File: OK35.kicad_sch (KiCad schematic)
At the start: 74 parts, among them SW1 SW_SPST, SW10 SW_SPST, SW11 SW_SPST, SW12 SW_SPST, SW13 SW_SPST, SW14 SW_SPST, SW15 SW_SPST, SW16 SW_SPST, SW17 SW_SPST, SW18 SW_SPST, SW19 SW_SPST, SW2 SW_SPST, SW20 SW_SPST, SW21 SW_SPST, SW22 SW_SPST, SW23 SW_SPST, SW24 SW_SPST, SW25 SW_SPST, SW26 SW_SPST, SW27 SW_SPST, SW28 SW_SPST, SW29 SW_SPST, SW3 SW_SPST, SW30 SW_SPST, SW31 SW_SPST, SW32 SW_SPST, SW33 SW_SPST, SW34 SW_SPST, SW35 SW_SPST, SW4 SW_SPST, SW5 SW_SPST, SW6 SW_SPST, SW7 SW_SPST, SW8 SW_SPST, SW9 SW_SPST, U1 TRRS, U2 ProMicro

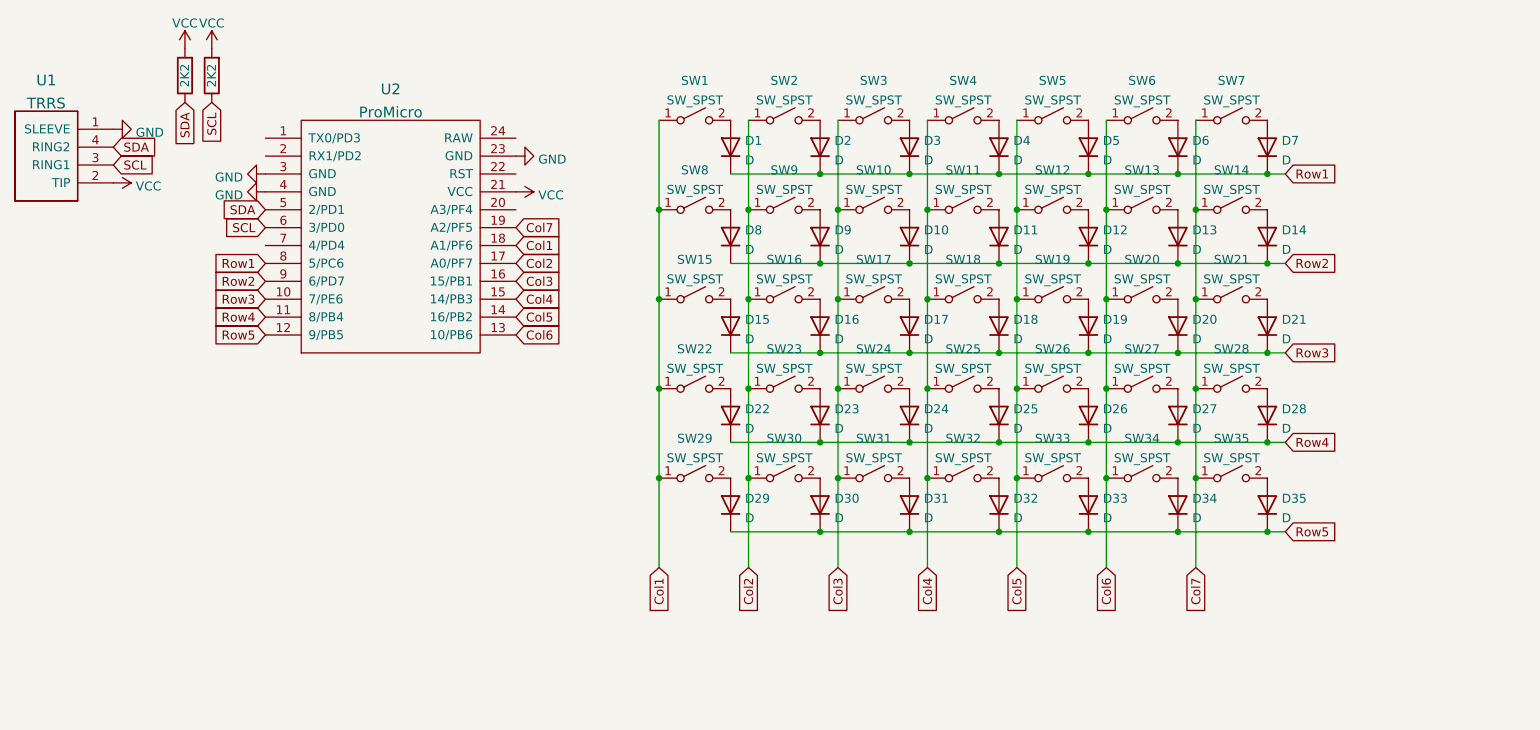
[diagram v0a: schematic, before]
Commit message: Add files via upload
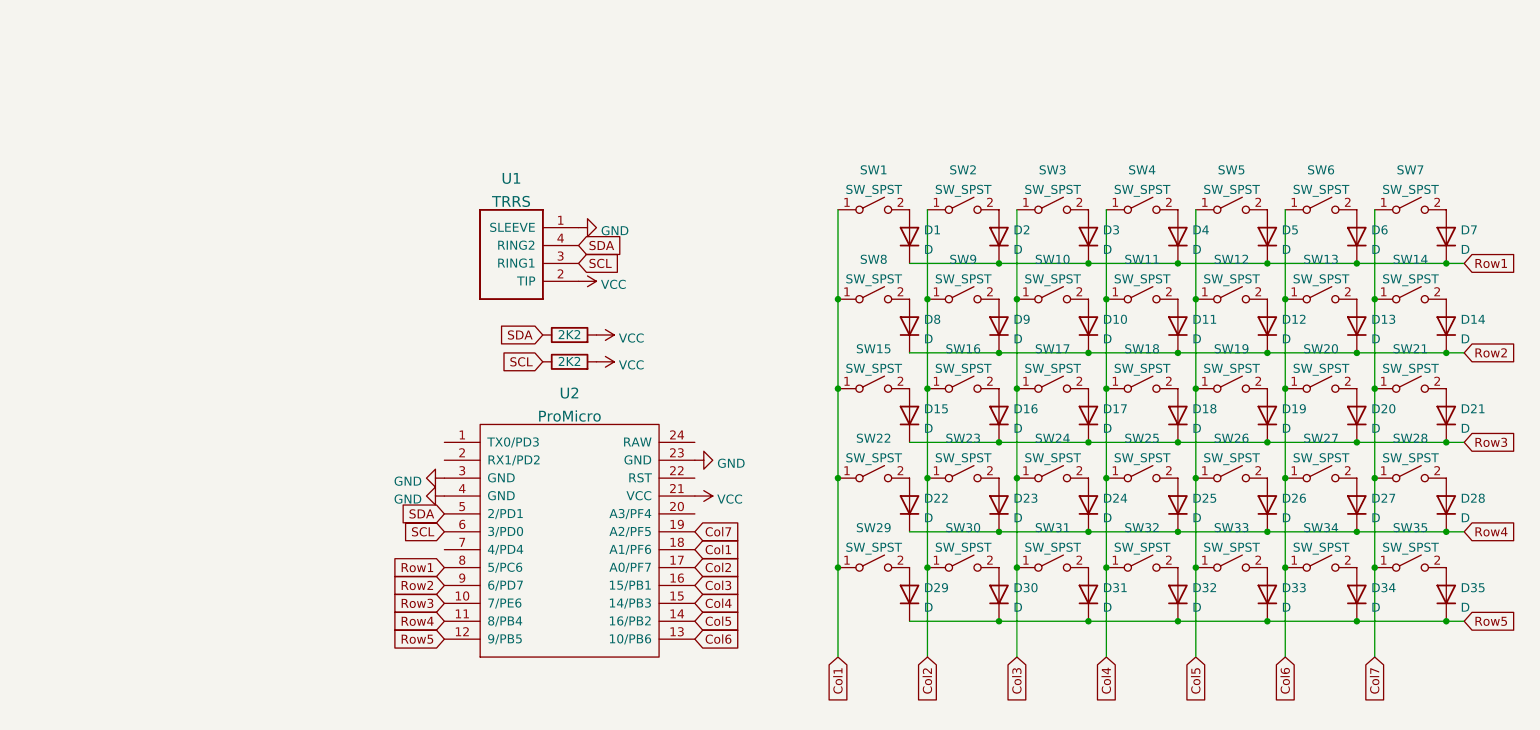
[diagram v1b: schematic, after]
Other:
- moved on the sheet: D1, D10, D11, D12, D13, D14, D15, D16, D17, D18, D19, D2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
